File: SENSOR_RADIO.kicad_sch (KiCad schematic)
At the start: 11 parts, among them U4 MCP602

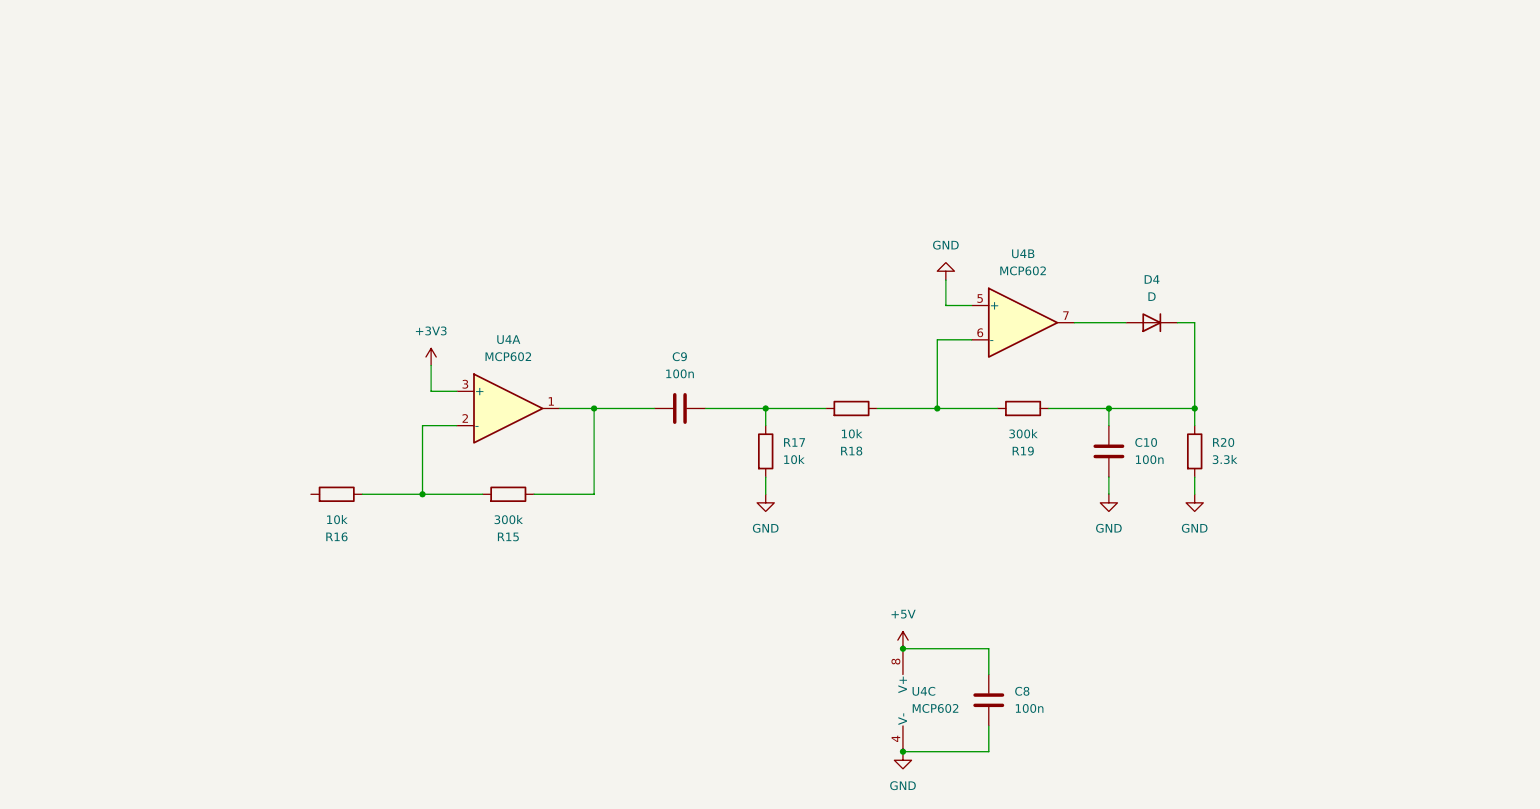
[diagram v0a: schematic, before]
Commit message: aaa
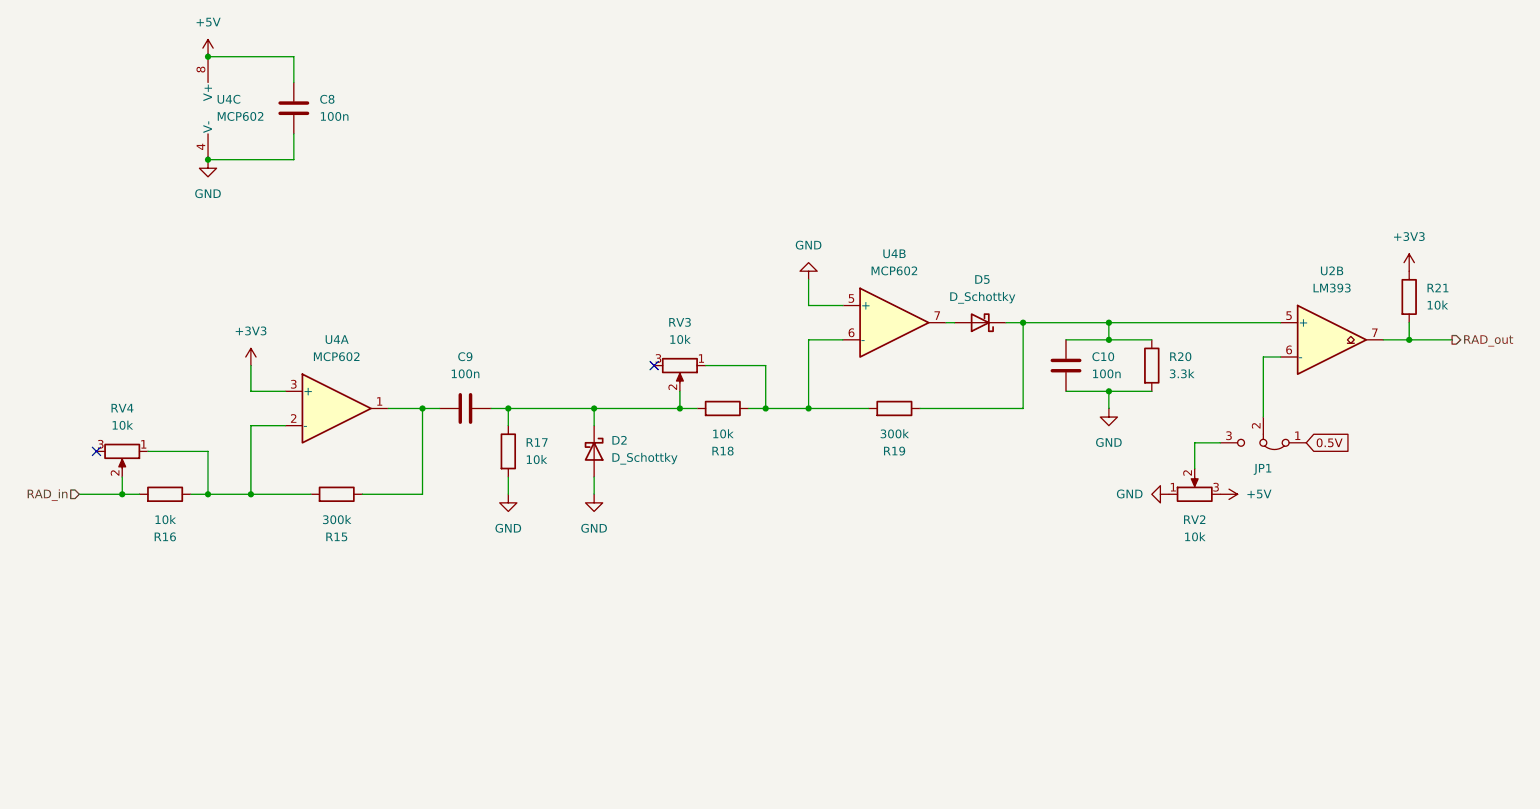
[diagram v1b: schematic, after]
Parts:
- removed D4: D, symbol Device:D
- added D2, D5: D_Schottky, Diode_SMD:D_SOD-123, symbol Device:D_Schottky
- added JP1: Jumper_3_Bridged12, Jumper:SolderJumper-3_P1.3mm_Bridged12_RoundedPad1.0x1.5mm_NumberLabels, symbol Jumper:Jumper_3_Bridged12
- added R21: 10k, Resistor_SMD:R_0805_2012Metric, symbol Device:R
- added RV2, RV3, RV4: 10k, symbol Device:R_Potentiometer
- added U2: LM393, Package_SO:SOIC-8_3.9x4.9mm_P1.27mm, symbol Comparator:LM393
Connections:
- net +3V3: now also R21.1
- net +5V: now also RV2.3
- net GND: now also D2.2 (A), RV2.1
- net at R15.2, R16.1, U4.2 (-): now also RV4.1
- net at C9.2, R17.1, R18.2: now also D2.1 (K), RV3.2
- net at R18.1, R19.2, U4.6 (-): now also RV3.1
- net at U4.7: now also D5.2 (A)
- net at C10.2, R19.1, R20.1: now also D5.1 (K), U2.5 (+)
- net RAD_in: now reaches R16.2
- net RAD_in: now also RV4.2
- new net: JP1.2 (C), U2.6 (-)
- new net: JP1.3 (B), RV2.2
- new net 0.5V: JP1.1 (A)
- new net RAD_out: R21.2, U2.7
- no-connect marks 0 -> 2
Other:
- moved on the sheet: C10, C8, C9, R15, R16, R17, R18, R19, R20, U4A, U4B, U4C

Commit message: aaa
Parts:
- RV2, RV3, RV4: footprint (none) -> Potentiometer_SMD:Potentiometer_Bourns_TC33X_Vertical
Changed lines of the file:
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@@
 			)
 		)
-		(property "Footprint" ""
+		(property "Footprint" "Potentiometer_SMD:Potentiometer_Bourns_TC33X_Vertical"
 			(at 209.55 107.95 0)
 			(effects
@@
 			)
 		)
-		(property "Footprint" ""
+		(property "Footprint" "Potentiometer_SMD:Potentiometer_Bourns_TC33X_Vertical"
 			(at 50.8 101.6 0)
 			(effects
@@
 			)
 		)
-		(property "Footprint" ""
+		(property "Footprint" "Potentiometer_SMD:Potentiometer_Bourns_TC33X_Vertical"
 			(at 133.35 88.9 0)
 			(effects
